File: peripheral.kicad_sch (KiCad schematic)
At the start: 26 parts, among them J1 JTAG, J2 UART_PROG, J3 Micro_SD_Card_Det_Hirose_DM3AT, J4 USB_MAIN, J5 USB_DBG, SW1 BOOT, SW2 RST

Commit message: Assign footprint
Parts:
- J4, J5: footprint (none) -> Connector_USB:USB_C_Receptacle_HRO_TYPE-C-31-M-12
- R5, R6: footprint (none) -> Resistor_SMD:R_0402_1005Metric
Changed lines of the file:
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@@
 			)
 		)
-		(property "Footprint" ""
+		(property "Footprint" "Resistor_SMD:R_0402_1005Metric"
 			(at 219.71 124.968 90)
 			(effects
@@
 			)
 		)
-		(property "Footprint" ""
+		(property "Footprint" "Connector_USB:USB_C_Receptacle_HRO_TYPE-C-31-M-12"
 			(at 52.07 147.32 0)
 			(effects
@@
 			)
 		)
-		(property "Footprint" ""
+		(property "Footprint" "Resistor_SMD:R_0402_1005Metric"
 			(at 219.71 123.952 90)
 			(effects
@@
 			)
 		)
-		(property "Footprint" ""
+		(property "Footprint" "Connector_USB:USB_C_Receptacle_HRO_TYPE-C-31-M-12"
 			(at 181.61 63.5 0)
 			(effects

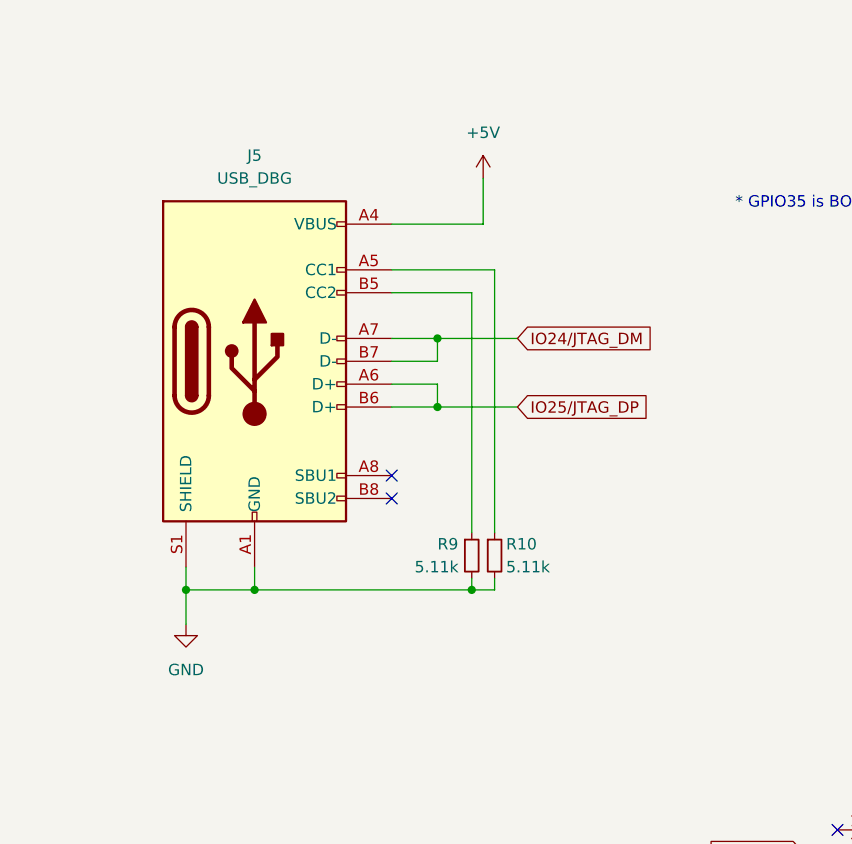
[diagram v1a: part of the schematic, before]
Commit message: Refine footprint matching
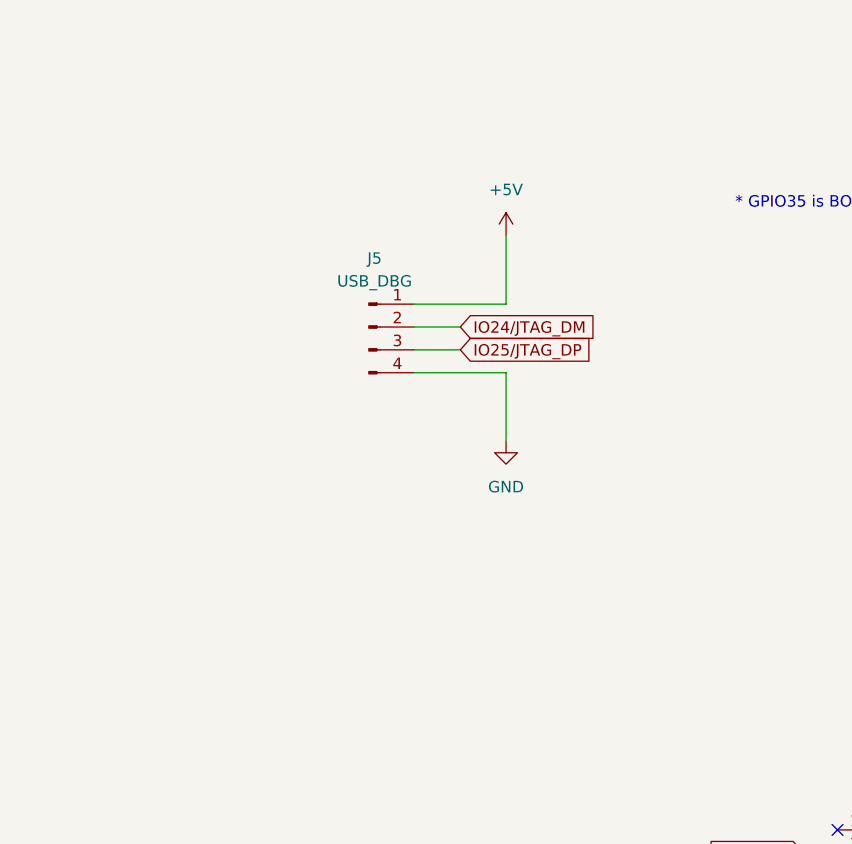
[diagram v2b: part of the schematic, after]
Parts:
- removed J5: USB_DBG, Connector_USB:USB_C_Receptacle_HRO_TYPE-C-31-M-12, symbol Connector:USB_C_Receptacle_USB2.0_16P
- removed R10, R9: 5.11k, Resistor_SMD:R_0402_1005Metric, symbol Device:R_Small
- added J5: USB_DBG, Connector_PinSocket_1.27mm:PinSocket_1x04_P1.27mm_Vertical, symbol Connector:Conn_01x04_Pin
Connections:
- net +5V: now also J5.1 (Pin_1)
- net GND: now also J5.4 (Pin_4)
- net IO24/JTAG_DM: now also J5.2 (Pin_2)
- net IO25/JTAG_DP: now also J5.3 (Pin_3)
- no-connect marks 5 -> 3

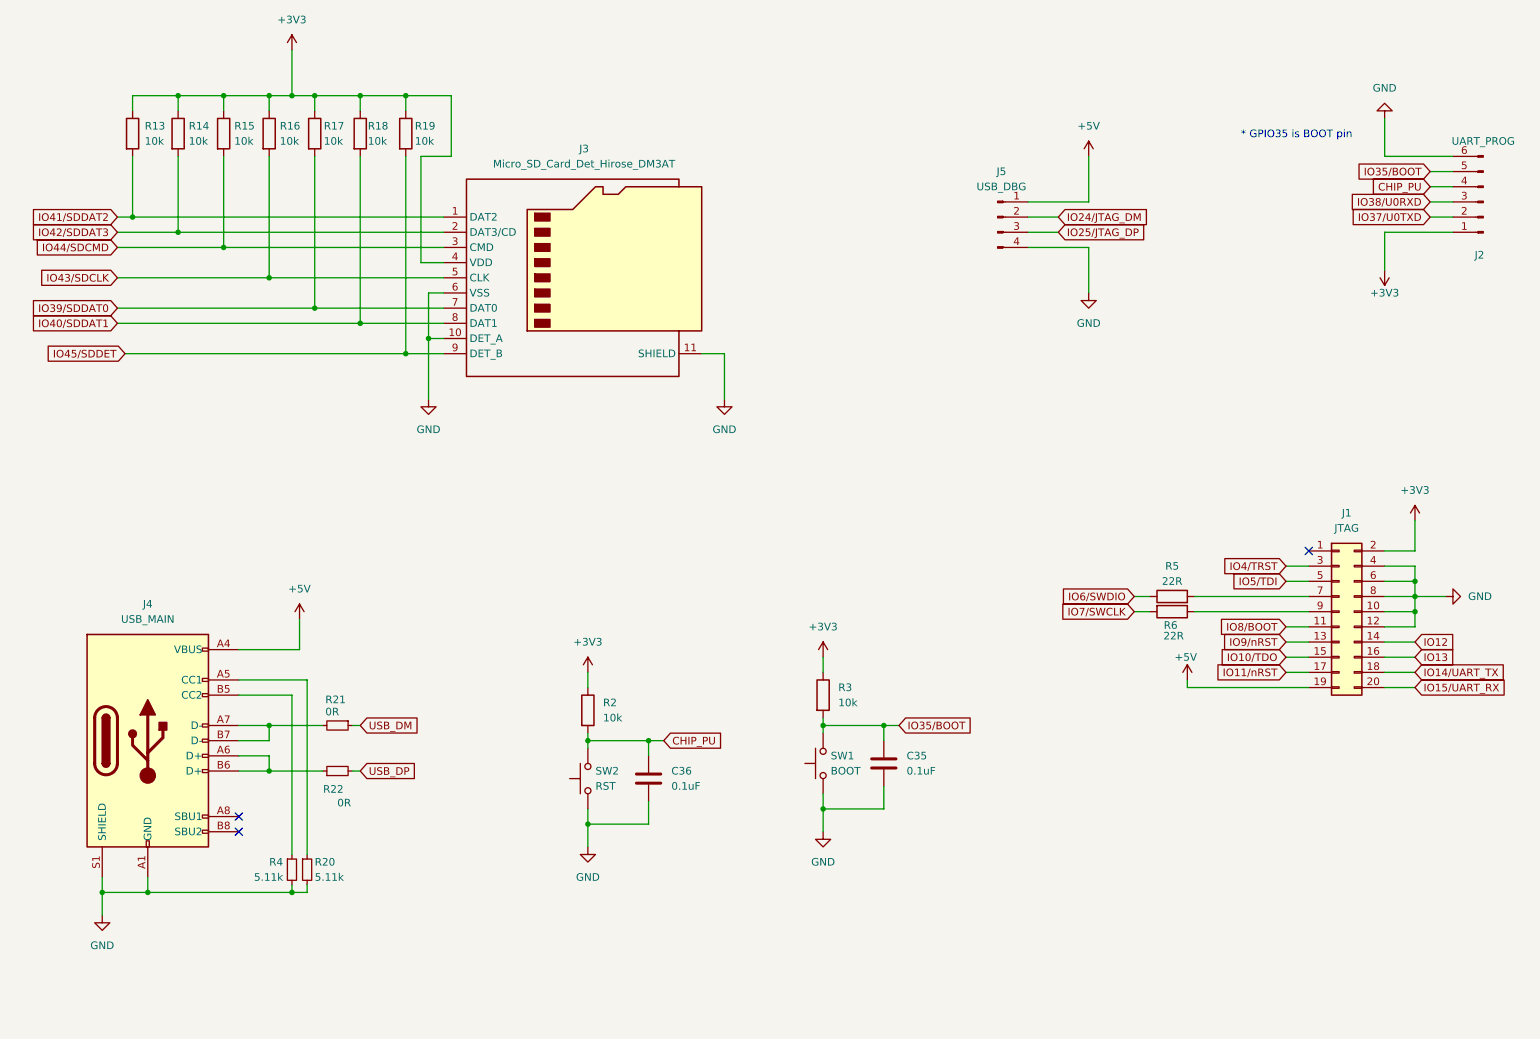
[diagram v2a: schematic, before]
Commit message: Rev 1
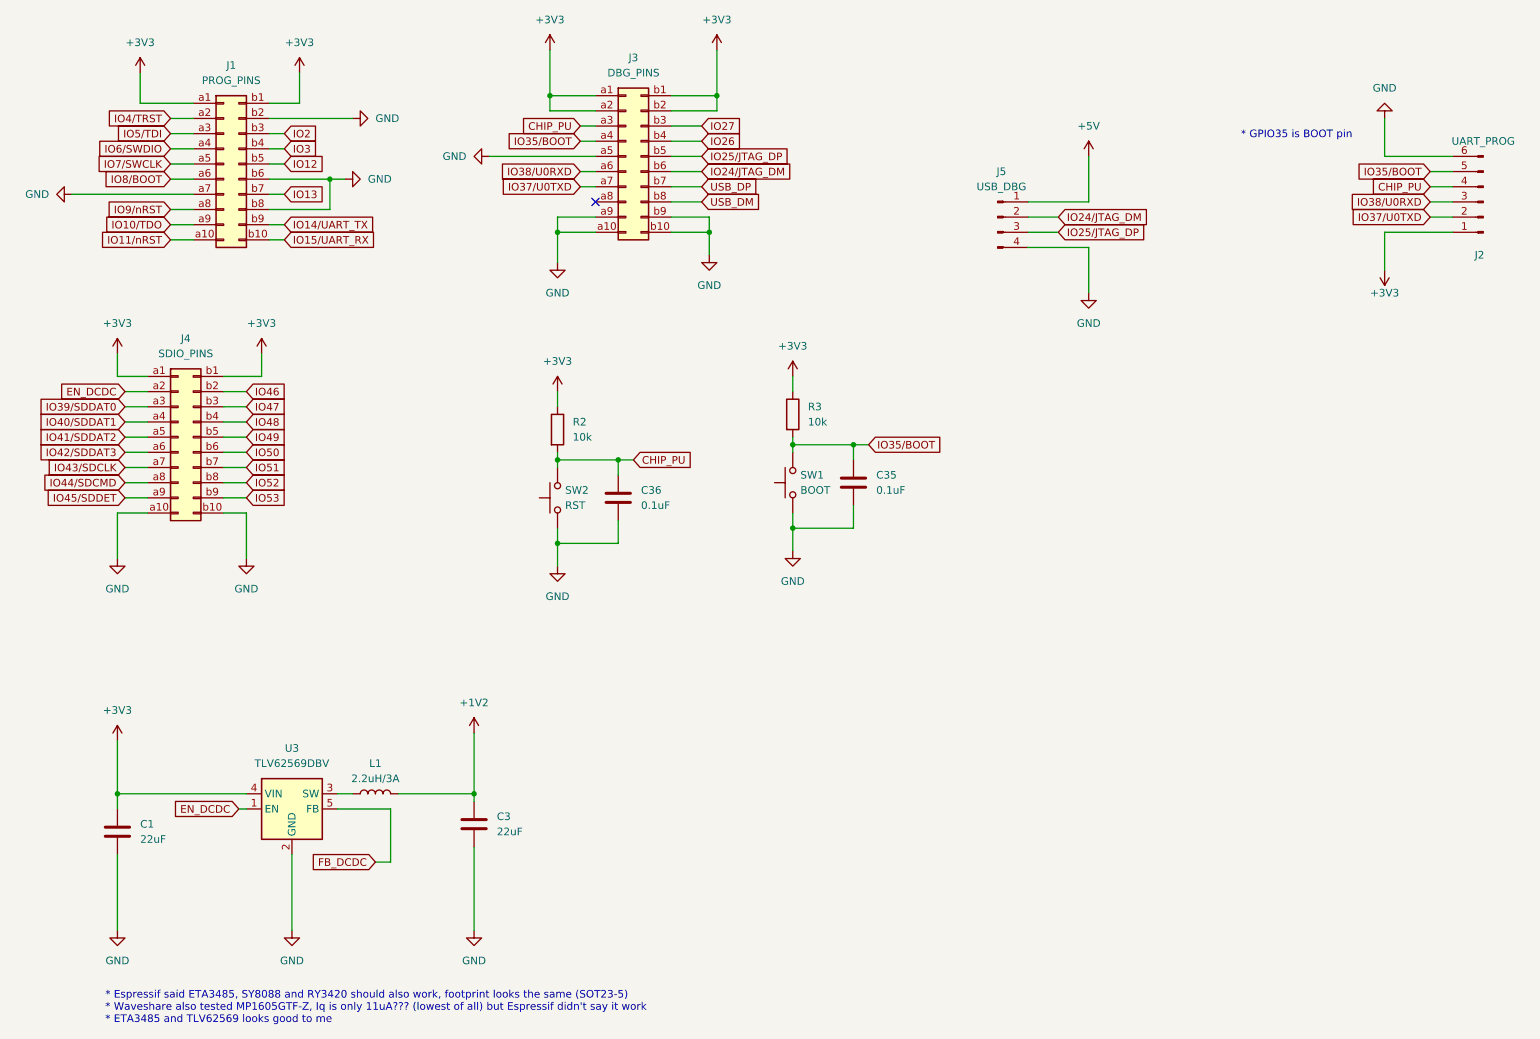
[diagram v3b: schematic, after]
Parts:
- removed J1: JTAG, Connector_PinHeader_2.54mm:PinHeader_2x10_P2.54mm_Vertical, symbol Connector_Generic:Conn_02x10_Odd_Even
- removed J3: Micro_SD_Card_Det_Hirose_DM3AT, Connector_Card:microSD_HC_Hirose_DM3AT-SF-PEJM5, symbol Connector:Micro_SD_Card_Det_Hirose_DM3AT
- removed J4: USB_MAIN, Connector_USB:USB_C_Receptacle_HRO_TYPE-C-31-M-12, symbol Connector:USB_C_Receptacle_USB2.0_16P
- removed R13, R14, R15, R16, R17, R18, R19: 10k, Resistor_SMD:R_0402_1005Metric, symbol Device:R
- removed R20, R4: 5.11k, Resistor_SMD:R_0402_1005Metric, symbol Device:R_Small
- removed R21, R22: 0R, Resistor_SMD:R_0402_1005Metric, symbol Device:R_Small
- removed R5, R6: 22R, Resistor_SMD:R_0402_1005Metric, symbol Device:R
- added C1, C3: 22uF, Capacitor_SMD:C_0402_1005Metric, symbol Device:C
- added J1: PROG_PINS, Connector_PinHeader_1.27mm:PinHeader_2x10_P1.27mm_Vertical_SMD, symbol Connector_Generic:Conn_02x10_Row_Letter_First
- added J3: DBG_PINS, Connector_PinHeader_1.27mm:PinHeader_2x10_P1.27mm_Vertical_SMD, symbol Connector_Generic:Conn_02x10_Row_Letter_First
- added J4: SDIO_PINS, Connector_PinHeader_1.27mm:PinHeader_2x10_P1.27mm_Vertical_SMD, symbol Connector_Generic:Conn_02x10_Row_Letter_First
- added L1: 2.2uH/3A, Inductor_SMD:L_Changjiang_FTC322510S, symbol Device:L
- added U3: TLV62569DBV, Package_TO_SOT_SMD:SOT-23-5, symbol Regulator_Switching:TLV62569DBV
- J2: footprint Connector_PinHeader_2.54mm:PinHeader_1x06_P2.54mm_Vertical -> Connector_PinHeader_1.27mm:PinHeader_1x06_P1.27mm_Vertical
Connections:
- net +3V3: now also C1.1, J1.a1 (Pin_a1), J1.b1 (Pin_b1), J3.a1 (Pin_a1), J3.a2 (Pin_a2), J3.b1 (Pin_b1), J3.b2 (Pin_b2), J4.a1 (Pin_a1), J4.b1 (Pin_b1), U3.4 (VIN)
- net CHIP_PU: now also J3.a3 (Pin_a3)
- net GND: now also C1.2, C3.2, J1.a7 (Pin_a7), J1.b2 (Pin_b2), J1.b6 (Pin_b6), J1.b8 (Pin_b8), J3.a10 (Pin_a10), J3.a5 (Pin_a5), J3.a9 (Pin_a9), J3.b10 (Pin_b10), J3.b9 (Pin_b9), J4.a10 (Pin_a10), J4.b10 (Pin_b10), U3.2 (GND)
- net IO10/TDO: now also J1.a9 (Pin_a9)
- net IO11/nRST: now also J1.a10 (Pin_a10)
- net IO12: now also J1.b5 (Pin_b5)
- net IO13: now also J1.b7 (Pin_b7)
- net IO14/UART_TX: now also J1.b9 (Pin_b9)
- net IO15/UART_RX: now also J1.b10 (Pin_b10)
- net IO24/JTAG_DM: now also J3.b6 (Pin_b6)
- net IO25/JTAG_DP: now also J3.b5 (Pin_b5)
- net IO35/BOOT: now also J3.a4 (Pin_a4)
- net IO37/U0TXD: now also J3.a7 (Pin_a7)
- net IO38/U0RXD: now also J3.a6 (Pin_a6)
- net IO39/SDDAT0: now also J4.a3 (Pin_a3)
- net IO40/SDDAT1: now also J4.a4 (Pin_a4)
- net IO41/SDDAT2: now also J4.a5 (Pin_a5)
- net IO42/SDDAT3: now also J4.a6 (Pin_a6)
- net IO43/SDCLK: now also J4.a7 (Pin_a7)
- net IO44/SDCMD: now also J4.a8 (Pin_a8)
- net IO45/SDDET: now also J4.a9 (Pin_a9)
- net IO4/TRST: now also J1.a2 (Pin_a2)
- net IO5/TDI: now also J1.a3 (Pin_a3)
- net IO6/SWDIO: now also J1.a4 (Pin_a4)
- net IO7/SWCLK: now also J1.a5 (Pin_a5)
- net IO8/BOOT: now also J1.a6 (Pin_a6)
- net IO9/nRST: now also J1.a8 (Pin_a8)
- net USB_DM: now also J3.b8 (Pin_b8)
- net USB_DP: now also J3.b7 (Pin_b7)
- new net: L1.1, U3.3 (SW)
- new net +1V2: C3.1, L1.2
- new net EN_DCDC: J4.a2 (Pin_a2), U3.1 (EN)
- new net FB_DCDC: U3.5 (FB)
- new net IO2: J1.b3 (Pin_b3)
- new net IO26: J3.b4 (Pin_b4)
- new net IO27: J3.b3 (Pin_b3)
- new net IO3: J1.b4 (Pin_b4)
- new net IO46: J4.b2 (Pin_b2)
- new net IO47: J4.b3 (Pin_b3)
- new net IO48: J4.b4 (Pin_b4)
- new net IO49: J4.b5 (Pin_b5)
- new net IO50: J4.b6 (Pin_b6)
- new net IO51: J4.b7 (Pin_b7)
- new net IO52: J4.b8 (Pin_b8)
- new net IO53: J4.b9 (Pin_b9)
- no-connect marks 3 -> 1
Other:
- note added: "* Espressif said ETA3485, SY8088 and RY3420 should also work, footprint looks the same (SOT23-5) * Waveshare also tested MP1605GTF-Z, Iq is only 11uA??? (lowest of all) but Espressif didn't say it work * ETA3485 and TLV62569 looks good to me"
- moved on the sheet: C35, C36, R2, R3, SW1, SW2
